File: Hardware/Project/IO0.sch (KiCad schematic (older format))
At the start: 2 parts, among them U15 74LS138, U6 8255

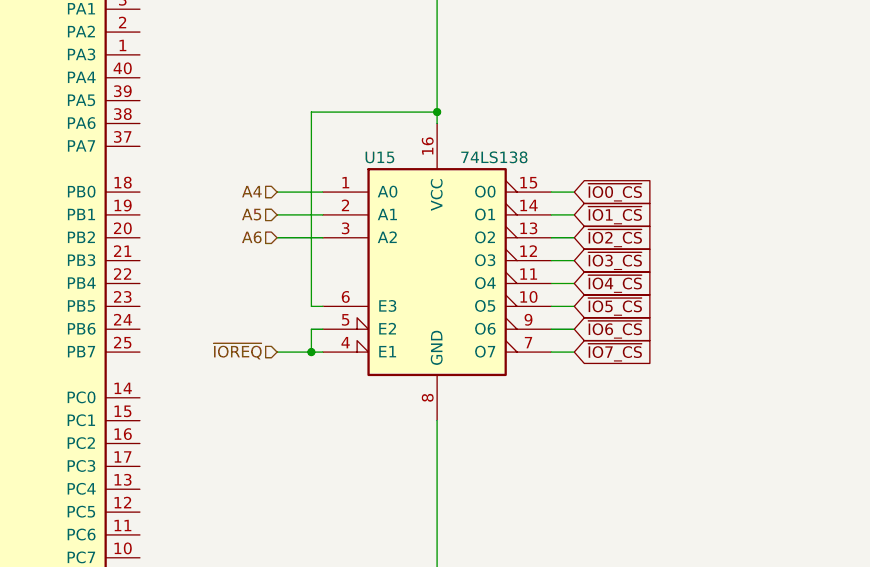
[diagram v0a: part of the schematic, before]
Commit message: 1
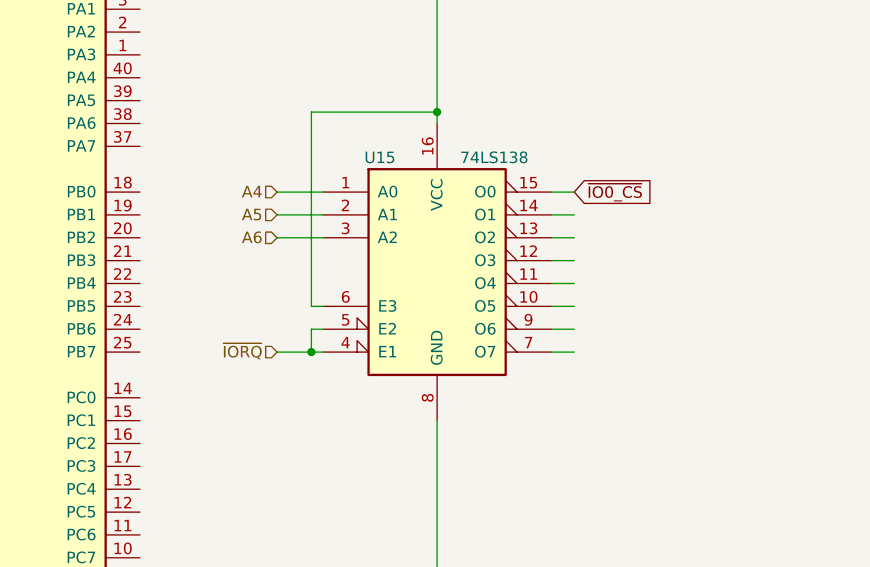
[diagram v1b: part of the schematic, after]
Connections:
- net labels added: ~IORQ
- net labels removed: ~IO1_CS, ~IO2_CS, ~IO3_CS, ~IO4_CS, ~IO5_CS, ~IO6_CS, ~IO7_CS, ~IOREQ
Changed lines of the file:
@@
 $Descr A3 16535 11693
 encoding utf-8
-Sheet 3 6
+Sheet 2 6
 Title ""
 Date ""
@@
 	5350 2700 5250 2700
 Text HLabel 4050 3400 0    50   Input ~ 0
-~IOREQ
+~IORQ
 Wire Wire Line
 	4050 3400 4200 3400
-Text GLabel 5350 2800 2    50   Input ~ 0
-~IO1_CS
 Wire Wire Line
 	5350 2800 5250 2800
-Text GLabel 5350 2900 2    50   Input ~ 0
-~IO2_CS
 Wire Wire Line
 	5350 2900 5250 2900
-Text GLabel 5350 3000 2    50   Input ~ 0
-~IO3_CS
 Wire Wire Line
 	5350 3000 5250 3000
-Text GLabel 5350 3100 2    50   Input ~ 0
-~IO4_CS
 Wire Wire Line
 	5350 3100 5250 3100
-Text GLabel 5350 3200 2    50   Input ~ 0
-~IO5_CS
 Wire Wire Line
 	5350 3200 5250 3200
-Text GLabel 5350 3300 2    50   Input ~ 0
-~IO6_CS
 Wire Wire Line
 	5350 3300 5250 3300
-Text GLabel 5350 3400 2    50   Input ~ 0
-~IO7_CS
 Wire Wire Line
 	5350 3400 5250 3400
